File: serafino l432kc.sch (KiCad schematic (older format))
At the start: 28 parts, among them J1 USB_B_Micro, J2 Conn_01x13, J3 Conn_01x13, Q1 AO3401A, SW1 SW_Push, SW2 SW_SPDT, U1 AP2112K-3.3, U2 USBLC6-2SC6, U3 STM32L432KCUx, Y1 32.768K

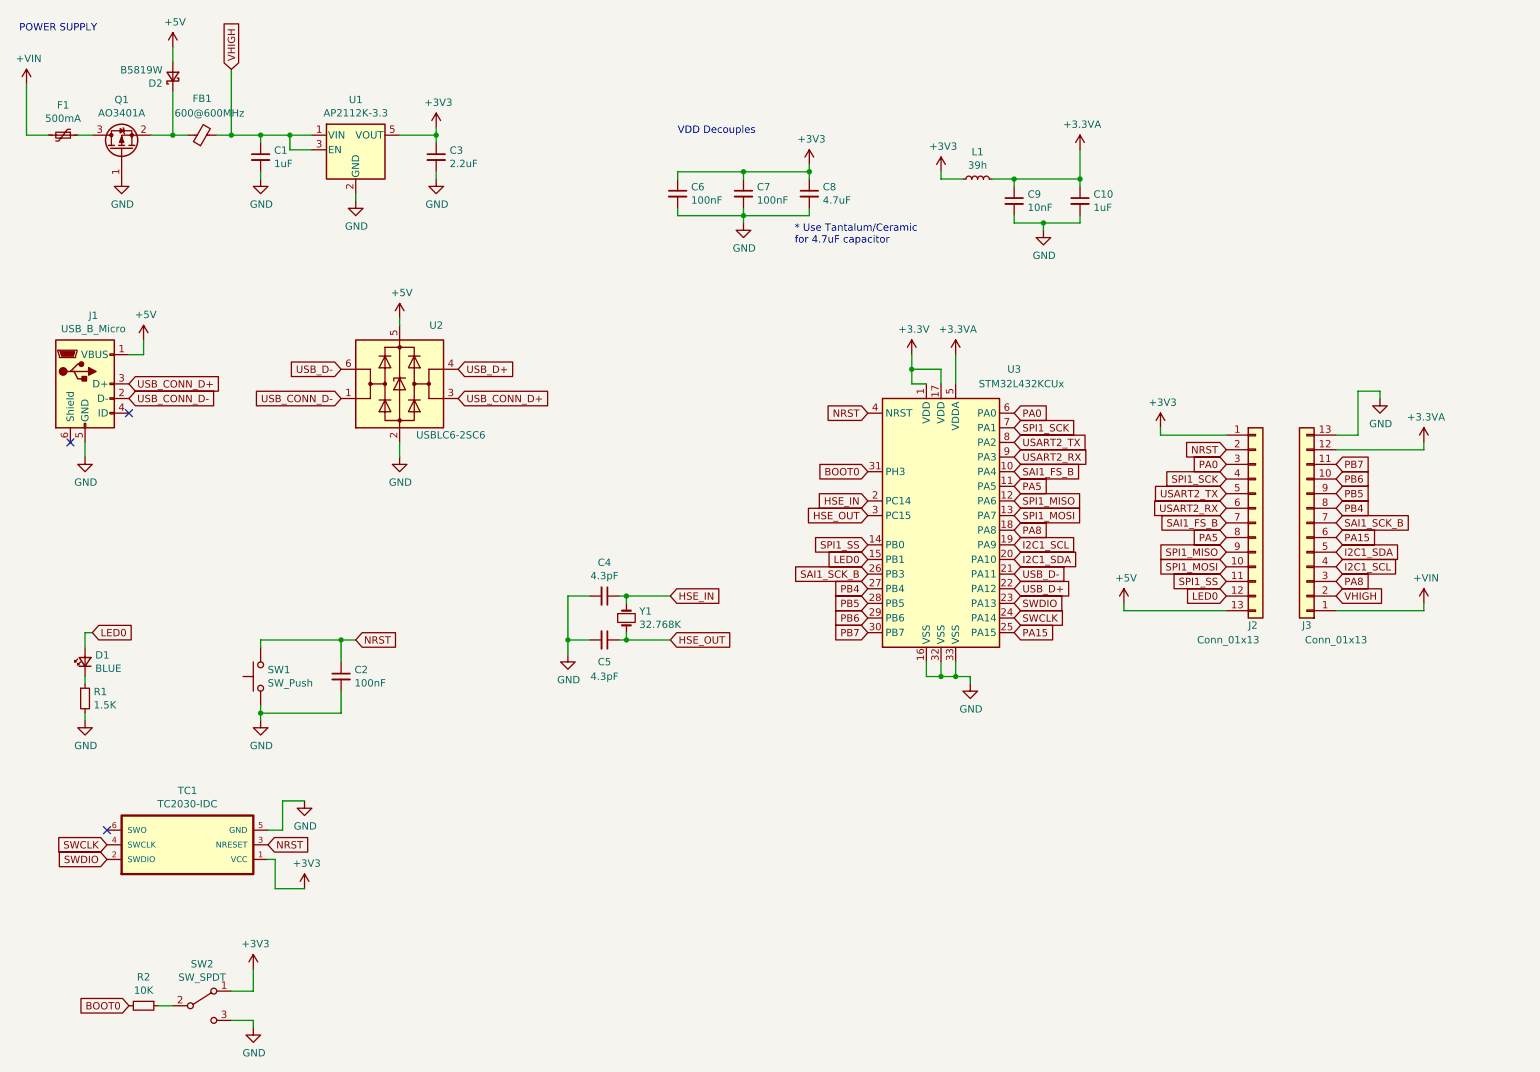
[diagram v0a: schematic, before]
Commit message: Layout avanzado...
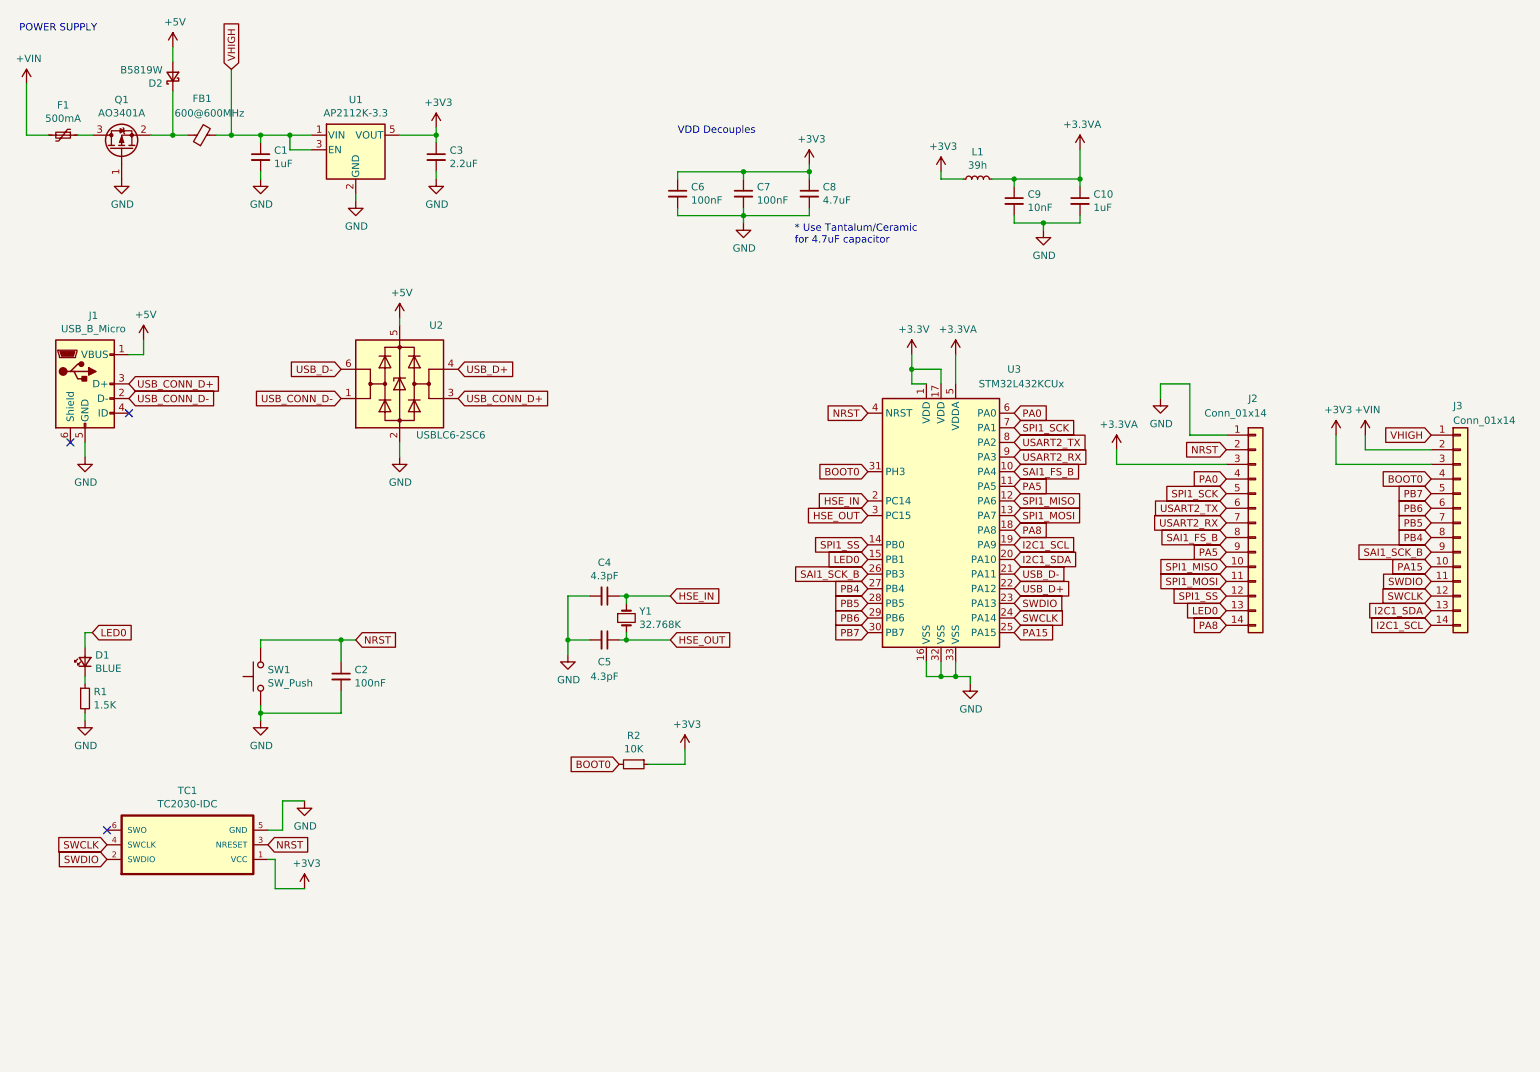
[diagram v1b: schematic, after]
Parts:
- removed J2, J3: Conn_01x13, Connector_PinHeader_2.54mm:PinHeader_1x13_P2.54mm_Vertical, symbol Connector_Generic:Conn_01x13
- removed SW2: SW_SPDT, Button_Switch_SMD:SW_DIP_SPSTx01_Slide_Copal_CHS-01A_W5.08mm_P1.27mm_JPin, symbol Switch:SW_SPDT
- added J2, J3: Conn_01x14, Connector_PinHeader_2.54mm:PinHeader_1x14_P2.54mm_Vertical, symbol Connector_Generic:Conn_01x14
- J1: footprint Connector_USB:USB_Micro-B_Molex-105017-0001 -> Connector_USB:USB_Micro-B_Molex-105133-0001
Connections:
- net +3.3VA: now also J2.3 (Pin_3)
- net +3V3: now also R2.1, J3.3 (Pin_3)
- net +VIN: now also J3.2 (Pin_2)
- net BOOT0: now also J3.4 (Pin_4)
- net GND: now also J2.1 (Pin_1)
- net I2C1_SCL: now also J3.14 (Pin_14)
- net I2C1_SDA: now also J3.13 (Pin_13)
- net LED0: now also J2.13 (Pin_13)
- net NRST: now also J2.2 (Pin_2)
- net PA0: now also J2.4 (Pin_4)
- net PA15: now also J3.10 (Pin_10)
- net PA5: now also J2.9 (Pin_9)
- net PA8: now also J2.14 (Pin_14)
- net PB4: now also J3.8 (Pin_8)
- net PB5: now also J3.7 (Pin_7)
- net PB6: now also J3.6 (Pin_6)
- net PB7: now also J3.5 (Pin_5)
- net SAI1_FS_B: now also J2.8 (Pin_8)
- net SAI1_SCK_B: now also J3.9 (Pin_9)
- net SPI1_MISO: now also J2.10 (Pin_10)
- net SPI1_MOSI: now also J2.11 (Pin_11)
- net SPI1_SCK: now also J2.5 (Pin_5)
- net SPI1_SS: now also J2.12 (Pin_12)
- net SWCLK: now also J3.12 (Pin_12)
- net SWDIO: now also J3.11 (Pin_11)
- net USART2_RX: now also J2.7 (Pin_7)
- net USART2_TX: now also J2.6 (Pin_6)
- net VHIGH: now also J3.1 (Pin_1)
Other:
- moved on the sheet: R2
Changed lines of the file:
@@
 	1    0    0    -1
 $EndComp
-$Comp
-L Switch:SW_SPDT SW2
-U 1 1 5FC70032
-P 1950 7350
-F 0 "SW2" H 1950 7635 50  0000 C CNN
-F 1 "SW_SPDT" H 1950 7544 50  0000 C CNN
-F 2 "Button_Switch_SMD:SW_DIP_SPSTx01_Slide_Copal_CHS-01A_W5.08mm_P1.27mm_JPin" H 1950 7350 50  0001 C CNN
-F 3 "~" H 1950 7350 50  0001 C CNN
-	1    1950 7350
-	1    0    0    -1
-$EndComp
-$Comp
-L Device:R_Small R2
-U 1 1 5FC716B0
-P 1550 7350
-F 0 "R2" V 1354 7350 50  0000 C CNN
-F 1 "10K" V 1445 7350 50  0000 C CNN
-F 2 "Resistor_SMD:R_0603_1608Metric" H 1550 7350 50  0001 C CNN
-F 3 "~" H 1550 7350 50  0001 C CNN
-	1    1550 7350
-	0    1    1    0
-$EndComp
-Text GLabel 1450 7350 0    50   Input ~ 0
-BOOT0
-Wire Wire Line
-	1650 7350 1750 7350
-$Comp
-L power:+3V3 #PWR016
-U 1 1 5FC7868A
-P 2300 7100
-F 0 "#PWR016" H 2300 6950 50  0001 C CNN
-F 1 "+3V3" H 2315 7273 50  0000 C CNN
-F 2 "" H 2300 7100 50  0001 C CNN
-F 3 "" H 2300 7100 50  0001 C CNN
-	1    2300 7100
-	1    0    0    -1
-$EndComp
-Wire Wire Line
-	2300 7100 2300 7250
-Wire Wire Line
-	2300 7250 2150 7250
 Text GLabel 6500 3900 0    50   Input ~ 0
 HSE_IN
@@
 F 0 "J1" H 1207 3567 50  0000 C CNN
 F 1 "USB_B_Micro" H 1207 3476 50  0000 C CNN
-F 2 "Connector_USB:USB_Micro-B_Molex-105017-0001" H 1300 3050 50  0001 C CNN
+F 2 "Connector_USB:USB_Micro-B_Molex-105133-0001" H 1300 3050 50  0001 C CNN
 F 3 "~" H 1300 3050 50  0001 C CNN
 	1    1150 3100
@@
 L power:GND #PWR0102
 U 1 1 5FE261BD
-P 10000 3200
-F 0 "#PWR0102" H 10000 2950 50  0001 C CNN
-F 1 "GND" H 10005 3027 50  0000 C CNN
-F 2 "" H 10000 3200 50  0001 C CNN
-F 3 "" H 10000 3200 50  0001 C CNN
-	1    10000 3200
+P 8500 3200
+F 0 "#PWR0102" H 8500 2950 50  0001 C CNN
+F 1 "GND" H 8505 3027 50  0000 C CNN
+F 2 "" H 8500 3200 50  0001 C CNN
+F 3 "" H 8500 3200 50  0001 C CNN
+	1    8500 3200
 	1    0    0    -1
 $EndComp
@@
 L power:+3V3 #PWR0103
 U 1 1 5FE29993
-P 8500 3400
-F 0 "#PWR0103" H 8500 3250 50  0001 C CNN
-F 1 "+3V3" H 8515 3573 50  0000 C CNN
-F 2 "" H 8500 3400 50  0001 C CNN
-F 3 "" H 8500 3400 50  0001 C CNN
-	1    8500 3400
+P 9700 3450
+F 0 "#PWR0103" H 9700 3300 50  0001 C CNN
+F 1 "+3V3" H 9715 3623 50  0000 C CNN
+F 2 "" H 9700 3450 50  0001 C CNN
+F 3 "" H 9700 3450 50  0001 C CNN
+	1    9700 3450
 	1    0    0    -1
 $EndComp
@@
 Connection ~ 7950 1700
 $Comp
-L power:+5V #PWR0106
-U 1 1 5FDF5F65
-P 8250 4600
-F 0 "#PWR0106" H 8250 4450 50  0001 C CNN
-F 1 "+5V" H 8265 4773 50  0000 C CNN
-F 2 "" H 8250 4600 50  0001 C CNN
-F 3 "" H 8250 4600 50  0001 C CNN
-	1    8250 4600
-	1    0    0    -1
-$EndComp
-$Comp
 L power:+3.3VA #PWR0107
 U 1 1 5FDF65C5
-P 10300 3500
-F 0 "#PWR0107" H 10300 3350 50  0001 C CNN
-F 1 "+3.3VA" H 10315 3673 50  0000 C CNN
-F 2 "" H 10300 3500 50  0001 C CNN
-F 3 "" H 10300 3500 50  0001 C CNN
-	1    10300 3500
-	1    0    0    -1
-$EndComp
-Text GLabel 9700 4350 2    50   Input ~ 0
+P 8200 3550
+F 0 "#PWR0107" H 8200 3400 50  0001 C CNN
+F 1 "+3.3VA" H 8215 3723 50  0000 C CNN
+F 2 "" H 8200 3550 50  0001 C CNN
+F 3 "" H 8200 3550 50  0001 C CNN
+	1    8200 3550
+	1    0    0    -1
+$EndComp
+Text GLabel 10350 4750 0    50   Input ~ 0
 I2C1_SCL
-Text GLabel 9700 4250 2    50   Input ~ 0
+Text GLabel 10350 4650 0    50   Input ~ 0
 I2C1_SDA
-Text GLabel 8950 3650 0    50   Input ~ 0
+Text GLabel 8950 3750 0    50   Input ~ 0
 PA0
 $Comp
 L power:+VIN #PWR0104
 U 1 1 5FD50E68
-P 10300 4600
-F 0 "#PWR0104" H 10300 4450 50  0001 C CNN
-F 1 "+VIN" H 10315 4773 50  0000 C CNN
-F 2 "" H 10300 4600 50  0001 C CNN
-F 3 "" H 10300 4600 50  0001 C CNN
-	1    10300 4600
-	1    0    0    -1
-$EndComp
-Text GLabel 9700 4550 2    50   Input ~ 0
+P 9900 3450
+F 0 "#PWR0104" H 9900 3300 50  0001 C CNN
+F 1 "+VIN" H 9915 3623 50  0000 C CNN
+F 2 "" H 9900 3450 50  0001 C CNN
+F 3 "" H 9900 3450 50  0001 C CNN
+	1    9900 3450
+	1    0    0    -1
+$EndComp
+Text GLabel 10350 3450 0    50   Input ~ 0
 VHIGH
 Text GLabel 8950 3550 0    50   Input ~ 0
 NRST
-Text GLabel 9700 4450 2    50   Input ~ 0
+Text GLabel 8950 4750 0    50   Input ~ 0
 PA8
-Text GLabel 9700 4150 2    50   Input ~ 0
+Text GLabel 10350 4350 0    50   Input ~ 0
 PA15
+Text GLabel 8950 4650 0    50   Input ~ 0
+LED0
 Text GLabel 8950 4550 0    50   Input ~ 0
-LED0
+SPI1_SS
+Text GLabel 10350 4250 0    50   Input ~ 0
+SAI1_SCK_B
+Text GLabel 10350 4150 0    50   Input ~ 0
+PB4
+Text GLabel 10350 4050 0    50   Input ~ 0
+PB5
+Text GLabel 10350 3950 0    50   Input ~ 0
+PB6
+Text GLabel 10350 3850 0    50   Input ~ 0
+PB7
 Text GLabel 8950 4450 0    50   Input ~ 0
-SPI1_SS
-Text GLabel 9700 4050 2    50   Input ~ 0
-SAI1_SCK_B
-Text GLabel 9700 3950 2    50   Input ~ 0
-PB4
-Text GLabel 9700 3850 2    50   Input ~ 0
-PB5
-Text GLabel 9700 3750 2    50   Input ~ 0
-PB6
-Text GLabel 9700 3650 2    50   Input ~ 0
-PB7
+SPI1_MOSI
 Text GLabel 8950 4350 0    50   Input ~ 0
-SPI1_MOSI
+SPI1_MISO
 Text GLabel 8950 4250 0    50   Input ~ 0
-SPI1_MISO
+PA5
 Text GLabel 8950 4150 0    50   Input ~ 0
-PA5
+SAI1_FS_B
 Text GLabel 8950 4050 0    50   Input ~ 0
-SAI1_FS_B
+USART2_RX
 Text GLabel 8950 3950 0    50   Input ~ 0
-USART2_RX
+USART2_TX
 Text GLabel 8950 3850 0    50   Input ~ 0
-USART2_TX
-Text GLabel 8950 3750 0    50   Input ~ 0
 SPI1_SCK
-$Comp
-L Connector_Generic:Conn_01x13 J2
-U 1 1 5FE0B8CC
-P 9150 4050
-F 0 "J2" H 9100 3350 50  0000 L CNN
-F 1 "Conn_01x13" H 8750 3250 50  0000 L CNN
-F 2 "Connector_PinHeader_2.54mm:PinHeader_1x13_P2.54mm_Vertical" H 9150 4050 50  0001 C CNN
-F 3 "~" H 9150 4050 50  0001 C CNN
-	1    9150 4050
-	1    0    0    -1
-$EndComp
-$Comp
-L Connector_Generic:Conn_01x13 J3
-U 1 1 5FE0CE9C
-P 9500 4050
-F 0 "J3" H 9500 4750 50  0000 C CNN
-F 1 "Conn_01x13" H 9300 4850 50  0000 C CNN
-F 2 "Connector_PinHeader_2.54mm:PinHeader_1x13_P2.54mm_Vertical" H 9500 4050 50  0001 C CNN
-F 3 "~" H 9500 4050 50  0001 C CNN
-	1    9500 4050
-	-1   0    0    1
-$EndComp
-Wire Wire Line
-	9850 3450 9700 3450
-Wire Wire Line
-	10300 4650 10300 4600
-Wire Wire Line
-	9700 4650 10300 4650
-Wire Wire Line
-	10300 3550 10300 3500
-Wire Wire Line
-	9700 3550 10300 3550
-Wire Wire Line
-	9850 3450 9850 3150
-Wire Wire Line
-	9850 3150 10000 3150
-Wire Wire Line
-	10000 3150 10000 3200
-Wire Wire Line
-	8500 3450 8500 3400
-Wire Wire Line
-	8500 3450 8950 3450
-Wire Wire Line
-	8950 4650 8250 4650
-Wire Wire Line
-	8250 4600 8250 4650
-$Comp
-L power:GND #PWR0108
-U 1 1 5FE71D91
-P 2300 7500
-F 0 "#PWR0108" H 2300 7250 50  0001 C CNN
-F 1 "GND" H 2305 7327 50  0000 C CNN
-F 2 "" H 2300 7500 50  0001 C CNN
-F 3 "" H 2300 7500 50  0001 C CNN
-	1    2300 7500
-	1    0    0    -1
-$EndComp
-Wire Wire Line
-	2300 7500 2300 7450
-Wire Wire Line
-	2300 7450 2150 7450
 Wire Wire Line
 	1750 800  1750 900
@@
 Wire Wire Line
 	2150 950  2150 1400
+Text GLabel 10350 4450 0    50   Input ~ 0
+SWDIO
+Text GLabel 10350 4550 0    50   Input ~ 0
+SWCLK
+$Comp
+L Connector_Generic:Conn_01x14 J3
+U 1 1 5FDF83D0
+P 10550 4050
+F 0 "J3" H 10500 4850 50  0000 L CNN
+F 1 "Conn_01x14" H 10500 4750 50  0000 L CNN
+F 2 "Connector_PinHeader_2.54mm:PinHeader_1x14_P2.54mm_Vertical" H 10550 4050 50  0001 C CNN
+F 3 "~" H 10550 4050 50  0001 C CNN
+	1    10550 4050
+	1    0    0    -1
+$EndComp
+$Comp
+L Connector_Generic:Conn_01x14 J2
+U 1 1 5FDFB498
+P 9150 4050
+F 0 "J2" H 9100 4900 50  0000 L CNN
+F 1 "Conn_01x14" H 8800 4800 50  0000 L CNN
+F 2 "Connector_PinHeader_2.54mm:PinHeader_1x14_P2.54mm_Vertical" H 9150 4050 50  0001 C CNN
+F 3 "~" H 9150 4050 50  0001 C CNN
+	1    9150 4050
+	1    0    0    -1
+$EndComp
+Wire Wire Line
+	8950 3650 8200 3650
+Wire Wire Line
+	8200 3650 8200 3550
+Text GLabel 4800 5700 0    50   Input ~ 0
+BOOT0
+$Comp
+L power:+3V3 #PWR016
+U 1 1 5FC7868A
+P 5250 5600
+F 0 "#PWR016" H 5250 5450 50  0001 C CNN
+F 1 "+3V3" H 5265 5773 50  0000 C CNN
+F 2 "" H 5250 5600 50  0001 C CNN
+F 3 "" H 5250 5600 50  0001 C CNN
+	1    5250 5600
+	1    0    0    -1
+$EndComp
+$Comp
+L Device:R_Small R2
+U 1 1 5FC716B0
+P 4900 5700
+F 0 "R2" V 4704 5700 50  0000 C CNN
+F 1 "10K" V 4795 5700 50  0000 C CNN
+F 2 "Resistor_SMD:R_0603_1608Metric" H 4900 5700 50  0001 C CNN
+F 3 "~" H 4900 5700 50  0001 C CNN
+	1    4900 5700
+	0    1    1    0
+$EndComp
+Wire Wire Line
+	5250 5600 5250 5700
+Wire Wire Line
+	5000 5700 5250 5700
+Wire Wire Line
+	9900 3450 9900 3550
+Wire Wire Line
+	9900 3550 10350 3550
+Wire Wire Line
+	9700 3450 9700 3650
+Wire Wire Line
+	9700 3650 10350 3650
+Wire Wire Line
+	8500 3200 8500 3100
+Wire Wire Line
+	8500 3100 8700 3100
+Wire Wire Line
+	8700 3100 8700 3450
+Wire Wire Line
+	8700 3450 8950 3450
+Text GLabel 10350 3750 0    50   Input ~ 0
+BOOT0
 $EndSCHEMATC

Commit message: Added 3D models...
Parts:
- J1: footprint Connector_USB:USB_Micro-B_Molex-105133-0001 -> Connector_USB:USB_Micro-B_Molex-105017-0001
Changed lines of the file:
@@
 F 0 "J1" H 1207 3567 50  0000 C CNN
 F 1 "USB_B_Micro" H 1207 3476 50  0000 C CNN
-F 2 "Connector_USB:USB_Micro-B_Molex-105133-0001" H 1300 3050 50  0001 C CNN
+F 2 "Connector_USB:USB_Micro-B_Molex-105017-0001" H 1300 3050 50  0001 C CNN
 F 3 "~" H 1300 3050 50  0001 C CNN
 	1    1150 3100
